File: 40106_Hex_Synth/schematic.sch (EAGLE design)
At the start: 39 parts, among them J15 POWER_JACK, U1 CD40106BE

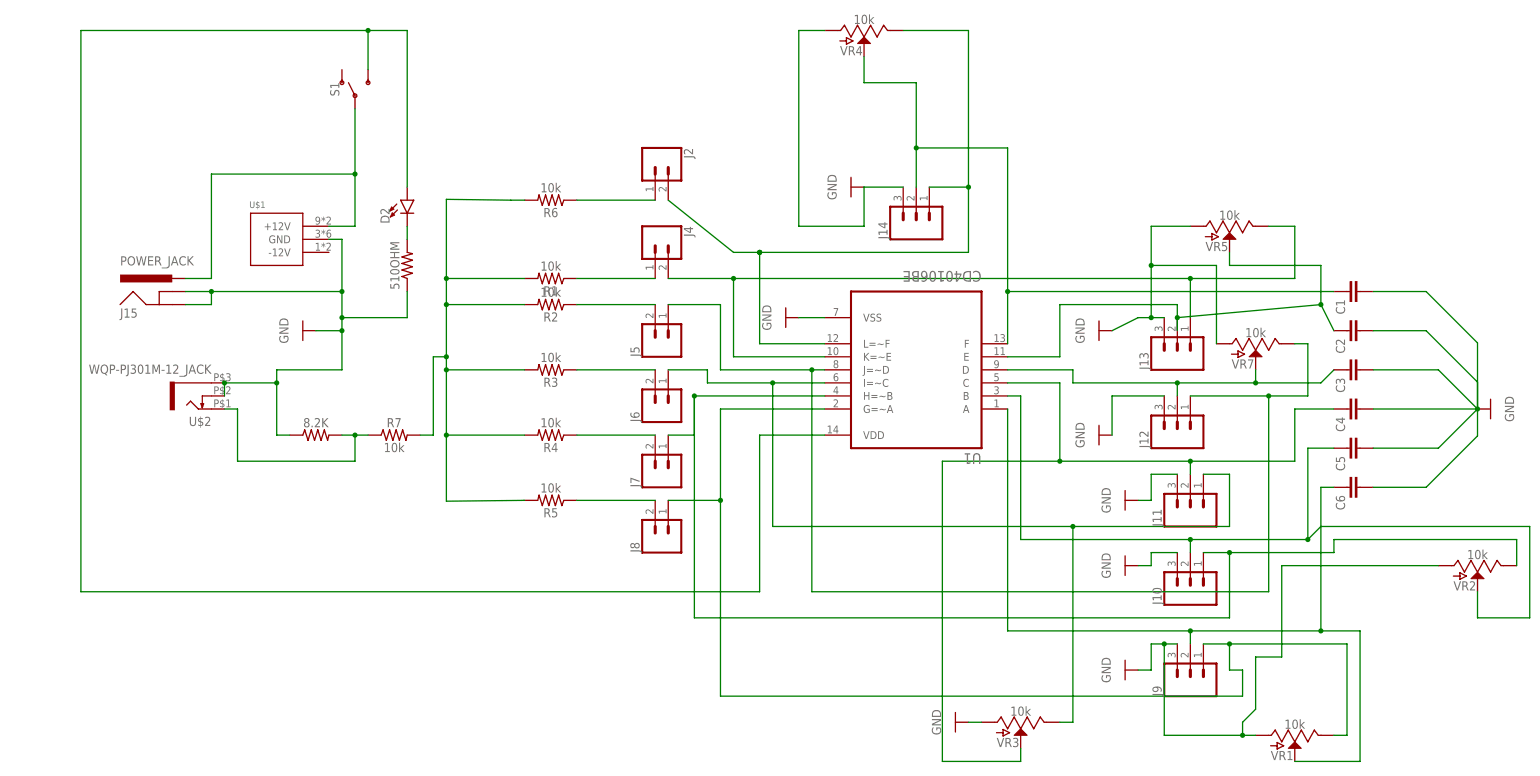
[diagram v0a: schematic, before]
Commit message: Add files via upload
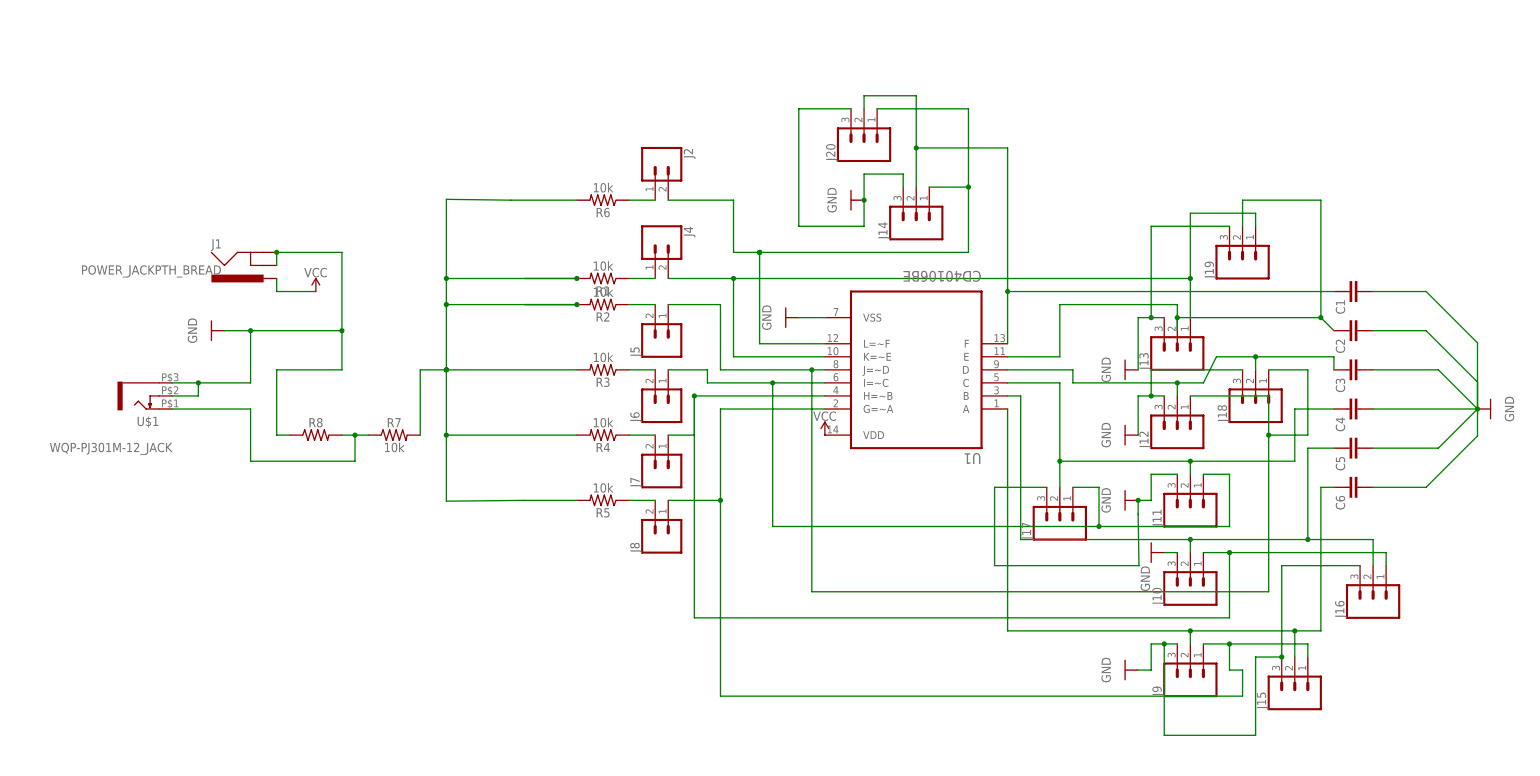
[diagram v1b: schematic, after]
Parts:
- removed 510OHM: (no value), SparkFun-Resistors:RESISTORAXIAL-0.3
- removed D2: (no value), SparkFun-LED:LED5MM
- removed S1: (no value), SparkFun-Switches:SWITCH-SPDT-PTH-11.6X4.0MM
- removed U$2: WQP-PJ301M-12_JACK, thonkiconn:WQP-PJ301M-12_JACK
- removed VR1, VR2, VR3, VR4, VR5, VR7: 10k, SparkFun-Resistors:POTENTIOMETER-PTH-9MM-1/20W-20%
- added J1: POWER_JACKPTH_BREAD, SparkFun-Connectors:POWER_JACKPTH_BREAD
- added J16, J17, J18, J19, J20: (no value), SparkFun-Connectors:CONN_03
- J15: value POWER_JACK -> (none); device SparkFun-Connectors:POWER_JACK -> SparkFun-Connectors:CONN_03
- U$1: value POWER_SIMPLE16 -> WQP-PJ301M-12_JACK; device eurorack:POWER_SIMPLE16 -> thonkiconn:WQP-PJ301M-12_JACK
- renumbered 8.2K to R8
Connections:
- removed net N$1 (its old number): 510OHM.2, D2.C
- removed net N$24: J15.PWR, S1.P, U$1.+12V
- removed net N$25: D2.A, S1.S, U1.VDD
- new net VCC: J1.PWR, U1.VDD
- net GND: now also J1.GND, J1.GNDBREAK, J15.3, J16.3, J17.3, J18.3, J19.3, J20.3, U$1.1, U$1.3; no longer 510OHM.1, J15.GND, J15.GNDBREAK, U$1.GND, U$2.1, U$2.3, VR1.A, VR2.A, VR3.A, VR4.A, VR5.A, VR7.A
- net N$15: now also J19.1; no longer VR5.E
- net N$16: now also J18.2; no longer VR7.S
- net N$17: now also J17.1; no longer VR3.E
- net N$18: now also J16.1; no longer VR2.E
- net N$19: now also J15.1; no longer VR1.E
- net N$2: now also J20.2; no longer VR4.S
- net N$21: now also U$1.2; no longer U$2.2
- net N$3: now also J20.1; no longer VR4.E
- net N$5: now also J18.1; no longer VR7.E
- net N$6: now also J17.2; no longer VR3.S
- net N$7: now also J16.2; no longer VR2.S
- net N$8: now also J15.2; no longer VR1.S
- net N$9: now also J19.2; no longer VR5.S
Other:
- moved on the sheet: R1, R2, R3, R4, R5, R6

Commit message: Add files via upload
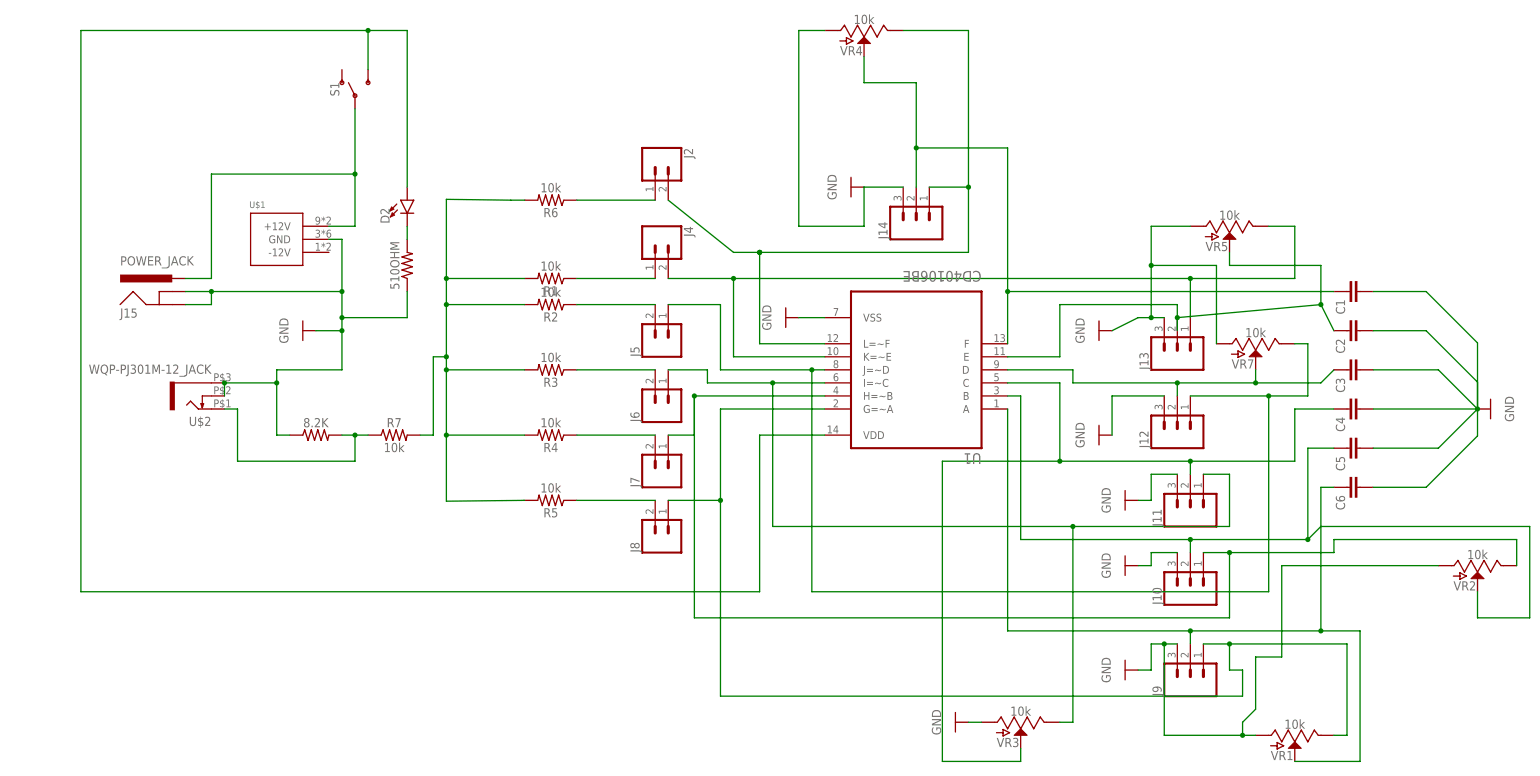
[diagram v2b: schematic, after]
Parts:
- removed J1: POWER_JACKPTH_BREAD, SparkFun-Connectors:POWER_JACKPTH_BREAD
- removed J16, J17, J18, J19, J20: (no value), SparkFun-Connectors:CONN_03
- added 510OHM: (no value), SparkFun-Resistors:RESISTORAXIAL-0.3
- added D2: (no value), SparkFun-LED:LED5MM
- added S1: (no value), SparkFun-Switches:SWITCH-SPDT-PTH-11.6X4.0MM
- added U$2: WQP-PJ301M-12_JACK, thonkiconn:WQP-PJ301M-12_JACK
- added VR1, VR2, VR3, VR4, VR5, VR7: 10k, SparkFun-Resistors:POTENTIOMETER-PTH-9MM-1/20W-20%
- J15: value (none) -> POWER_JACK; device SparkFun-Connectors:CONN_03 -> SparkFun-Connectors:POWER_JACK
- U$1: value WQP-PJ301M-12_JACK -> POWER_SIMPLE16; device thonkiconn:WQP-PJ301M-12_JACK -> eurorack:POWER_SIMPLE16
- renumbered R8 to 8.2K
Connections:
- removed net VCC: J1.PWR, U1.VDD
- new net N$1: 510OHM.2, D2.C
- new net N$24: J15.PWR, S1.P, U$1.+12V
- new net N$25: D2.A, S1.S, U1.VDD
- net GND: now also 510OHM.1, J15.GND, J15.GNDBREAK, U$1.GND, U$2.1, U$2.3, VR1.A, VR2.A, VR3.A, VR4.A, VR5.A, VR7.A; no longer J1.GND, J1.GNDBREAK, J15.3, J16.3, J17.3, J18.3, J19.3, J20.3, U$1.1, U$1.3
- net N$15: now also VR5.E; no longer J19.1
- net N$16: now also VR7.S; no longer J18.2
- net N$17: now also VR3.E; no longer J17.1
- net N$18: now also VR2.E; no longer J16.1
- net N$19: now also VR1.E; no longer J15.1
- net N$2: now also VR4.S; no longer J20.2
- net N$21: now also U$2.2; no longer U$1.2
- net N$3: now also VR4.E; no longer J20.1
- net N$5: now also VR7.E; no longer J18.1
- net N$6: now also VR3.S; no longer J17.2
- net N$7: now also VR2.S; no longer J16.2
- net N$8: now also VR1.S; no longer J15.2
- net N$9: now also VR5.S; no longer J19.2
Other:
- moved on the sheet: R1, R2, R3, R4, R5, R6
